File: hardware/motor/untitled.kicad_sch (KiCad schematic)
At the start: 88 parts, among them CN1 MR30PW-F, CN2 MR30PW-F, Q1 EMB09N03V, Q10 EMB09N03V, Q11 EMB09N03V, Q12 EMB09N03V, Q13 EMB09N03V, Q14 EMB09N03V, Q15 EMB09N03V, Q16 EMB09N03V, Q2 EMB09N03V, Q7 EMB09N03V, Q8 EMB09N03V, Q9 EMB09N03V, U1 EG2133, U2 EG2133

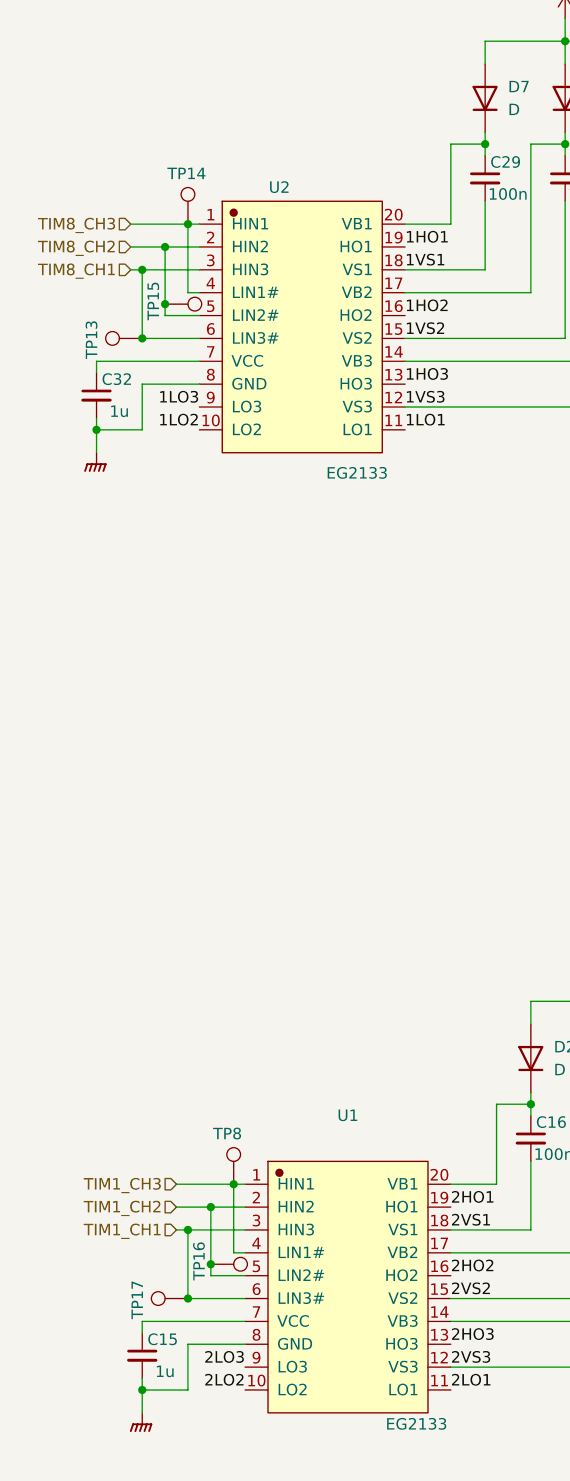
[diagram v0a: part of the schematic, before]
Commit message: update rfBat pcb
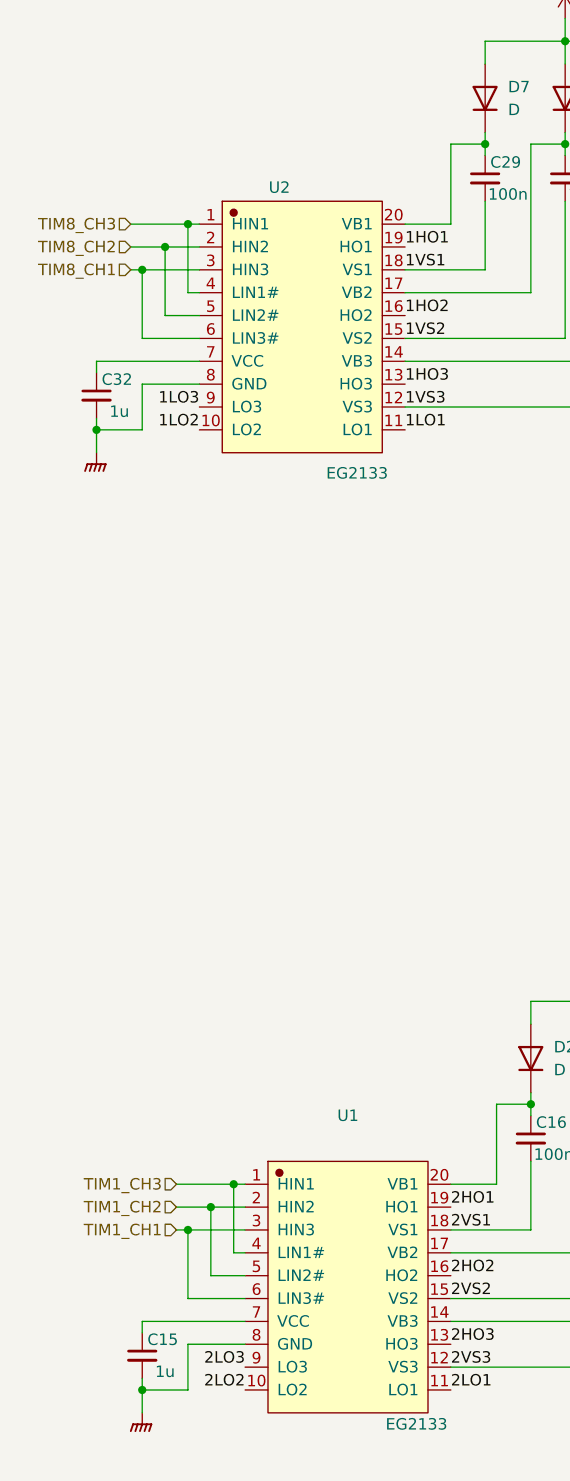
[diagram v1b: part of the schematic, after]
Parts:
- removed TP13, TP14, TP15, TP16, TP17, TP8: TestPoint, TestPoint:TestPoint_Pad_D1.0mm, symbol Connector:TestPoint

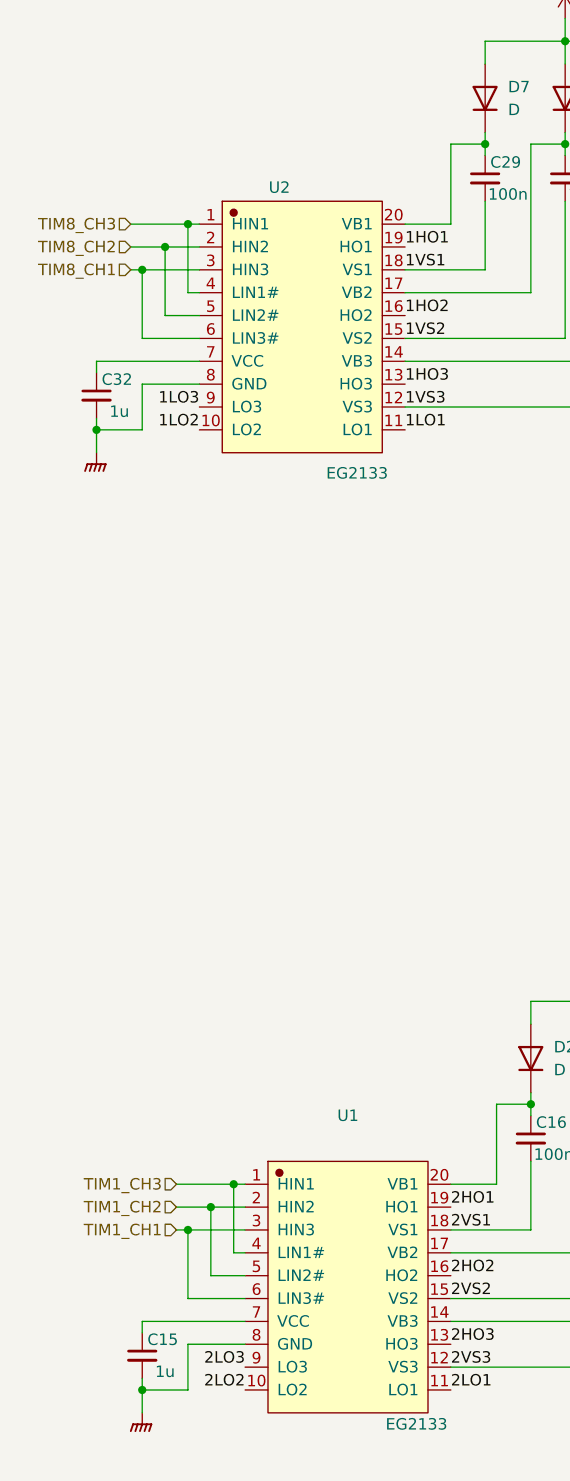
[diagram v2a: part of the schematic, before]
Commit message: update controller firmware
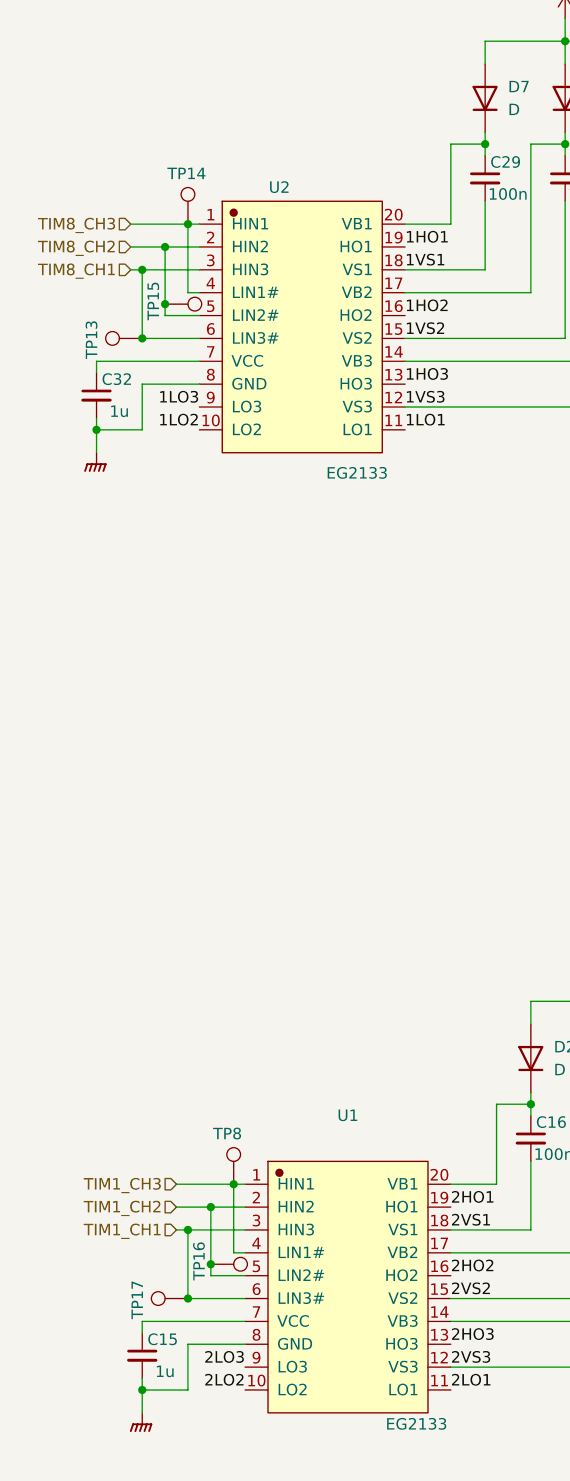
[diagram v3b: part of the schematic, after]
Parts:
- added TP13, TP14, TP15, TP16, TP17, TP8: TestPoint, TestPoint:TestPoint_Pad_D1.0mm, symbol Connector:TestPoint
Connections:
- net TIM1_CH1: now also TP17.1
- net TIM1_CH2: now also TP16.1
- net TIM1_CH3: now also TP8.1
- net TIM8_CH1: now also TP13.1
- net TIM8_CH2: now also TP15.1
- net TIM8_CH3: now also TP14.1
